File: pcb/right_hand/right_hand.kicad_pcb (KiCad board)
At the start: 2 copper layers, 160 x 110 mm, 113 parts, among them J0 UJ20-C-H-G-SMT-P16-TR, U0 SW_Push

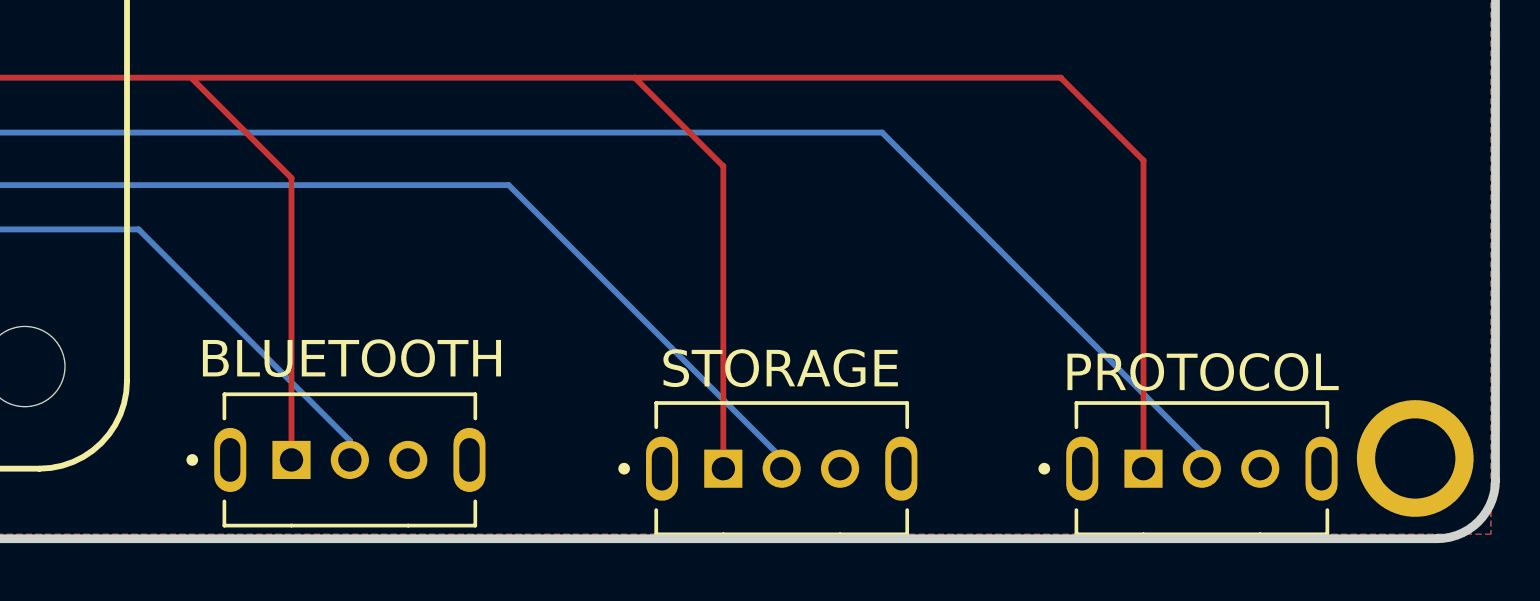
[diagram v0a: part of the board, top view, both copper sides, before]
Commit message: Fix Bluetooh Enable positioning
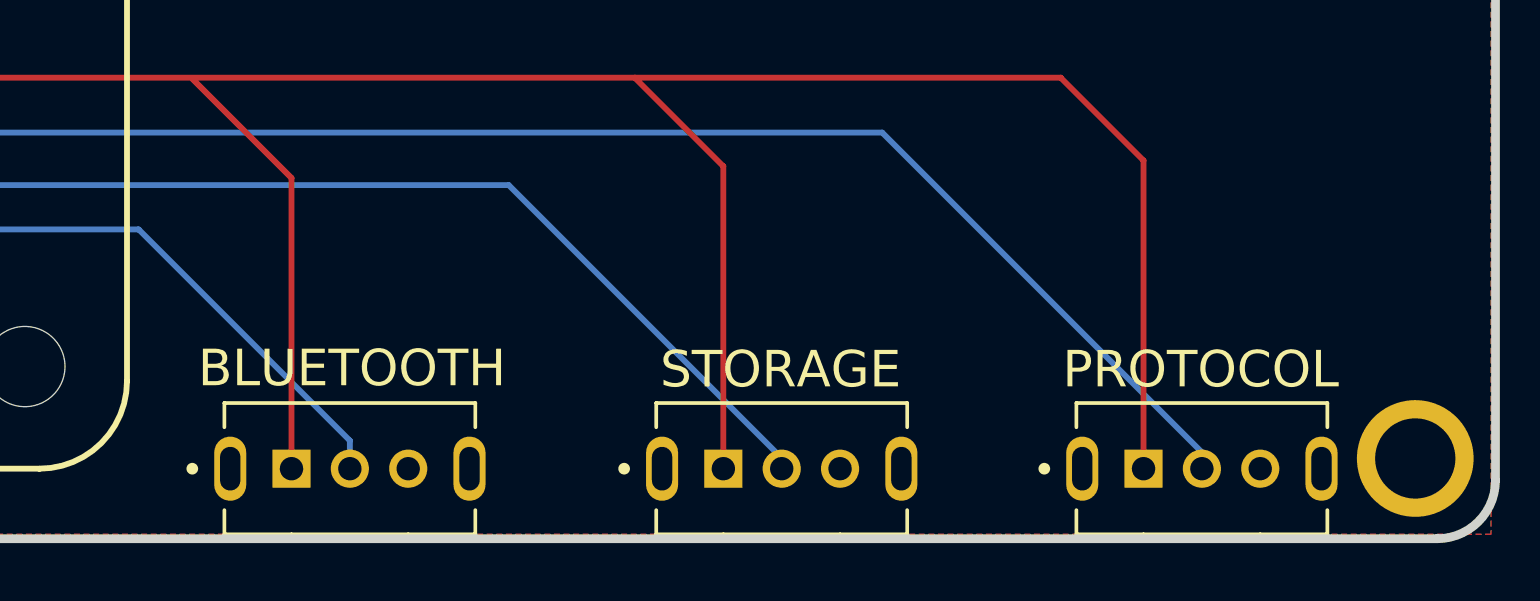
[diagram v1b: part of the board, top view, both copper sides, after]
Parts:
- moved BLUETOOTH 0.30 mm to (190.0, 144.6)
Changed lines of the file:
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@@
 		(at 219.2375 144.6)
 		(property "Reference" "PROTOCOL"
-			(at -0.0375 -3.27 0)
+			(at -0.0375 -3.4 0)
 			(layer "F.SilkS")
 			(effects
@@
 	(footprint "snap_magic_footprints:SW_SLW-864587-2A-RA-N-D"
 		(layer "F.Cu")
-		(at 190.0375 144.3)
+		(at 190.0375 144.6)
 		(property "Reference" "BLUETOOTH"
 			(at 0.0725 -3.44 0)
@@
 	)
 	(segment
+		(start 188.0375 144.6)
+		(end 188.0375 134.6375)
+		(width 0.2)
+		(layer "F.Cu")
+		(net 80)
+	)
+	(segment
 		(start 214.4 131.2)
 		(end 217.2375 134.0375)
@@
 	)
 	(segment
-		(start 188.0375 134.6375)
-		(end 188.0375 144.3)
-		(width 0.2)
-		(layer "F.Cu")
-		(net 80)
-	)
-	(segment
 		(start 217.2375 134.0375)
 		(end 217.2375 144.6)
@@
 	)
 	(segment
-		(start 182.8 136.4)
+		(start 190.0375 144.6)
 		(end 190.0375 143.6375)
 		(width 0.2)
@@
 	)
 	(segment
-		(start 190.0375 143.6375)
-		(end 190.0375 144.3)
+		(start 182.8 136.4)
+		(end 190.0375 143.6375)
 		(width 0.2)
 		(layer "B.Cu")
@@
 			)
 		)
+	)
+	(zone
+		(net 0)
+		(net_name "")
+		(layers "F.Cu" "B.Cu")
+		(hatch edge 0.5)
+		(connect_pads
+			(clearance 0)
+		)
+		(min_thickness 0.25)
+		(filled_areas_thickness no)
+		(keepout
+			(tracks allowed)
+			(vias allowed)
+			(pads allowed)
+			(copperpour not_allowed)
+			(footprints allowed)
+		)
+		(placement
+			(enabled no)
+			(sheetname "")
+		)
+		(fill
+			(thermal_gap 0.5)
+			(thermal_bridge_width 0.5)
+		)
+		(polygon
+			(pts
+				(xy 222.4 145.4) (xy 222.4 146.8) (xy 225.2 146.8) (xy 225.2 145.4)
+			)
+		)
